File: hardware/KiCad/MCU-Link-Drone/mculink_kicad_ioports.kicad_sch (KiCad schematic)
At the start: 8 parts, among them J3 Jumper_2_Open, J4 Jumper_2_Open, J5 Jumper_2_Open, SW1 KMR221GLFS, U1 LPC55S69JBD64

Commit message: improved layout
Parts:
- U1: footprint McuOnEclipse:LQFP-64-1EP_10x10mm_P0.5mm_EP5x5mm -> McuOnEclipse:LQFP-64-1EP_10x10mm_P0.5mm_EP3.5x3.5mm
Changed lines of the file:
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@@
 			)
 		)
-		(property "Footprint" "McuOnEclipse:LQFP-64-1EP_10x10mm_P0.5mm_EP5x5mm"
+		(property "Footprint" "McuOnEclipse:LQFP-64-1EP_10x10mm_P0.5mm_EP3.5x3.5mm"
 			(at 33.02 19.05 0)
 			(effects
@@
 			)
 		)
-		(property "Footprint" "McuOnEclipse:LQFP-64-1EP_10x10mm_P0.5mm_EP5x5mm"
+		(property "Footprint" "McuOnEclipse:LQFP-64-1EP_10x10mm_P0.5mm_EP3.5x3.5mm"
 			(at 33.02 86.36 0)
 			(effects

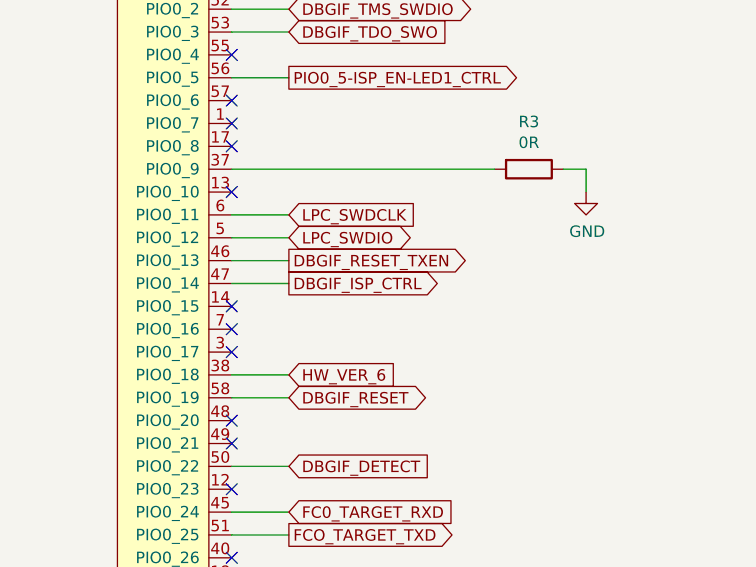
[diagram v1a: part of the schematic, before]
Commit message: optimized layout
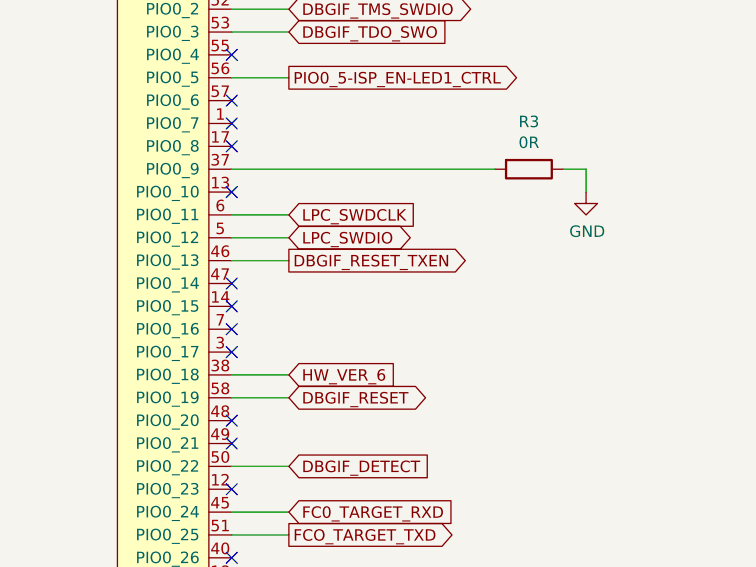
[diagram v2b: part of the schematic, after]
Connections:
- net DBGIF_ISP_CTRL: no longer names the net of U1.47 (PIO0_14)
- no-connect marks 18 -> 19
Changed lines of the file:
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@@
+	)
+	(no_connect
+		(at 44.45 63.5)
 	)
 	(no_connect
@@
 		(pts
 			(xy 50.8 60.96) (xy 44.45 60.96)
-		)
-		(stroke
-			(width 0)
-			(type default)
-		)
-	)
-	(wire
-		(pts
-			(xy 44.45 63.5) (xy 50.8 63.5)
 		)
 		(stroke
@@
 			(effects
 				(font
-					(size 1.27 1.27)
-				)
-				(hide yes)
-			)
-		)
-	)
-	(global_label "DBGIF_ISP_CTRL"
-		(shape output)
-		(at 50.8 63.5 0)
-		(effects
-			(font
-				(size 1.27 1.27)
-			)
-			(justify left)
-		)
-		(property "Intersheetrefs" "${INTERSHEET_REFS}"
-			(at 50.8 63.5 0)
-			(effects
-				(font
